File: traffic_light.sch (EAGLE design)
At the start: 31 parts, among them IC1 74LS48N, IC2 74LS48N, IC3 NE555N, IC6 74190N, IC7 74190N

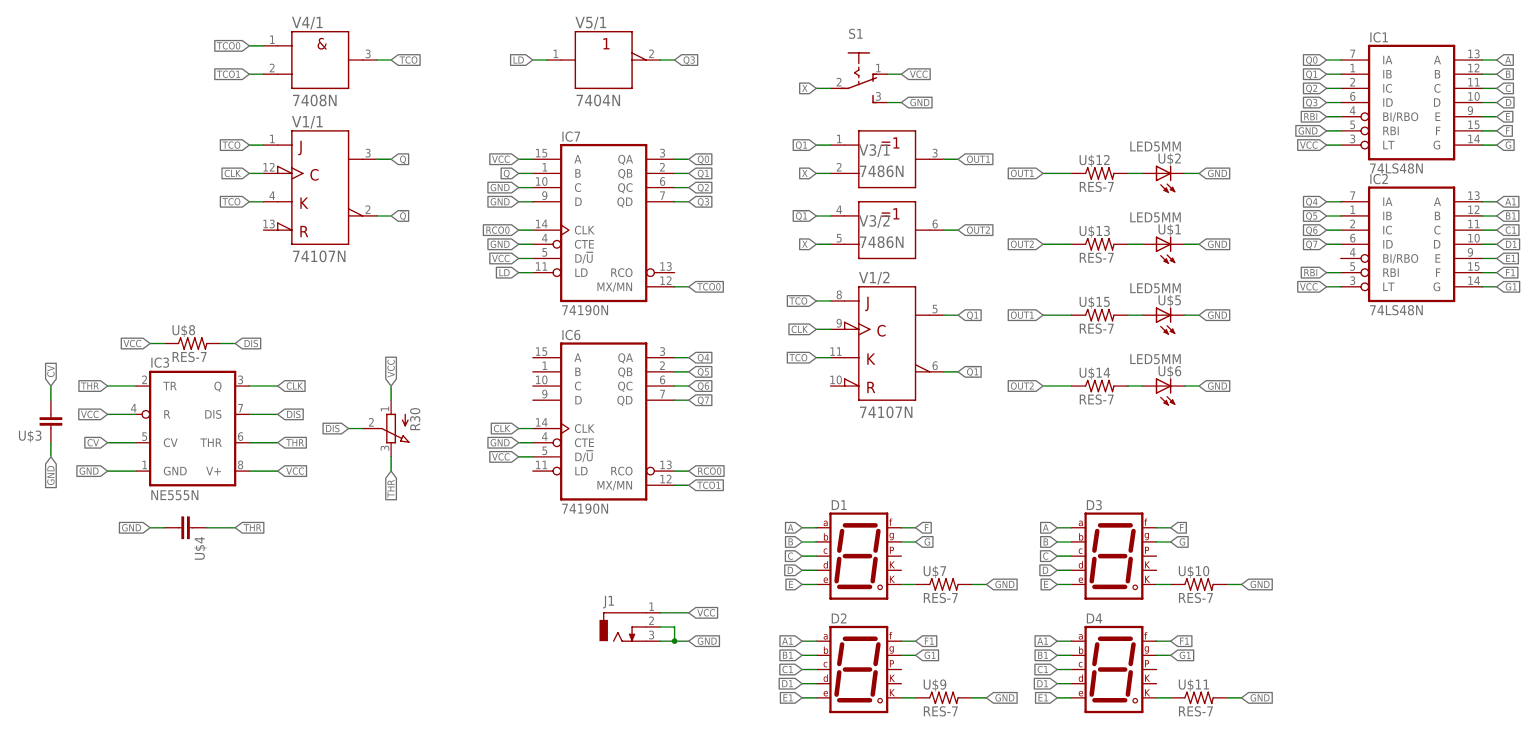
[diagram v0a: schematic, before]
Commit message: schematics
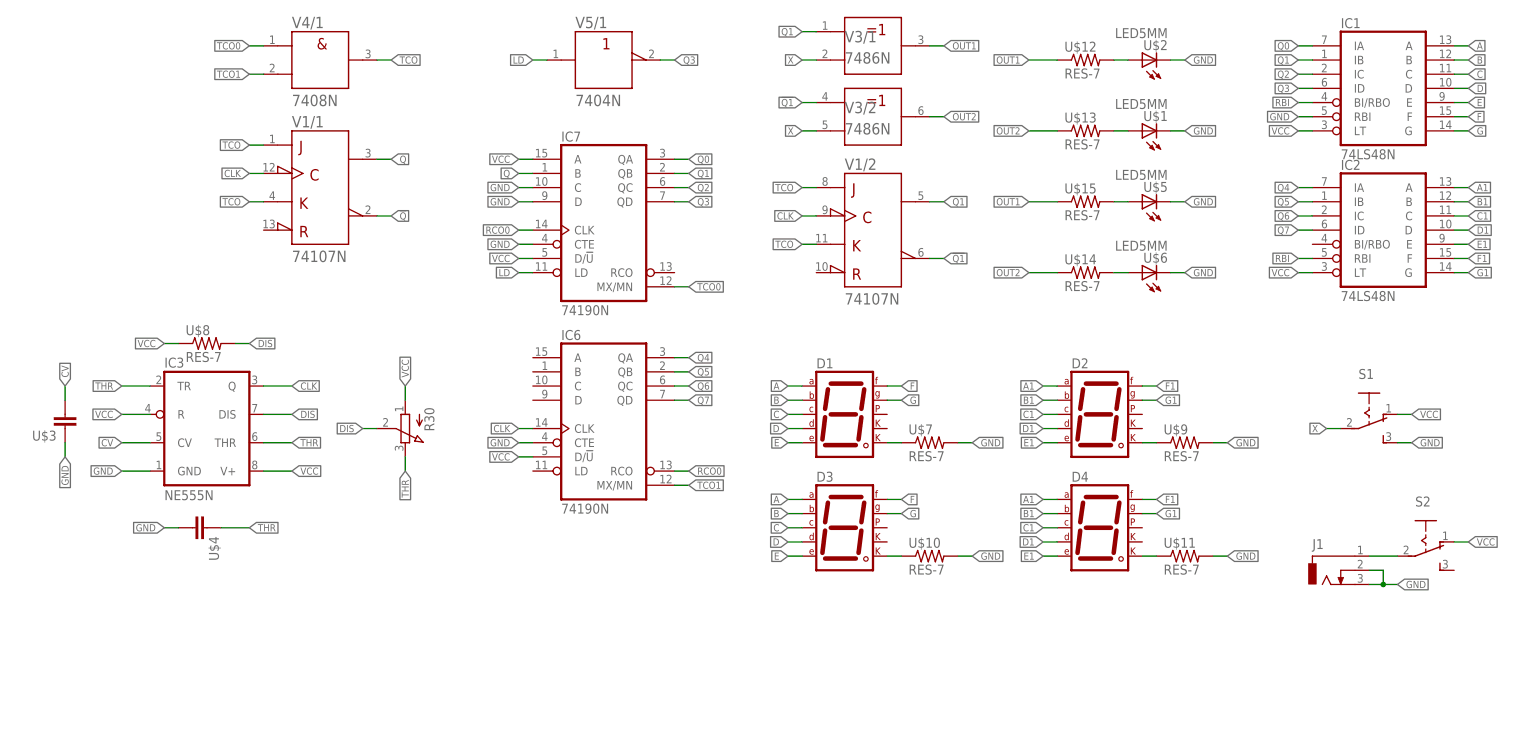
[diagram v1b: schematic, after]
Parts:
- added S2: (no value), switch:255SB
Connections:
- new net N$5: J1.1, S2.P
- net VCC: now also S2.O; no longer J1.1
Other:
- moved on the sheet: D1, D2, D3, D4, IC1, IC2, IC3, J1, R30, S1, U$1, U$10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
